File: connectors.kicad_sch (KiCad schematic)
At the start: 23 parts, among them J2 SM08B-SRSS-TB

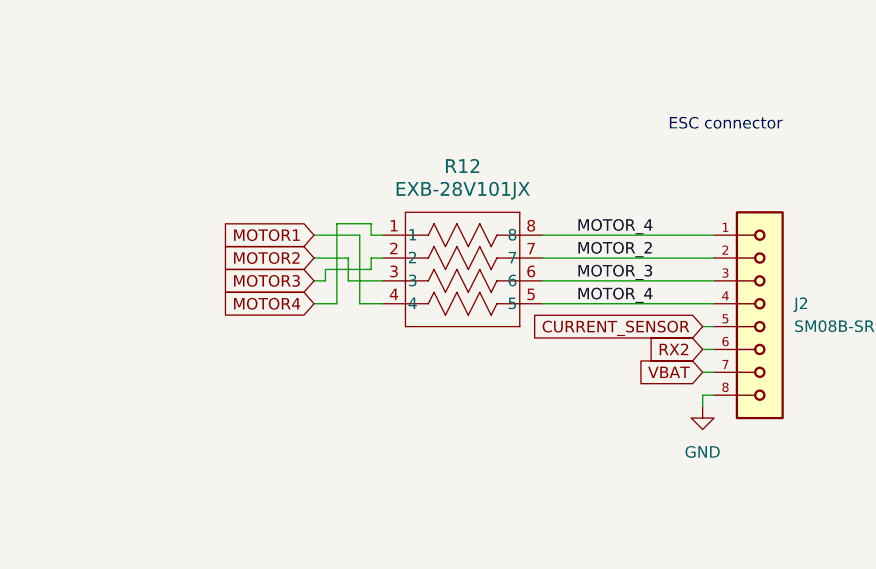
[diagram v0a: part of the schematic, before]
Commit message: routing...
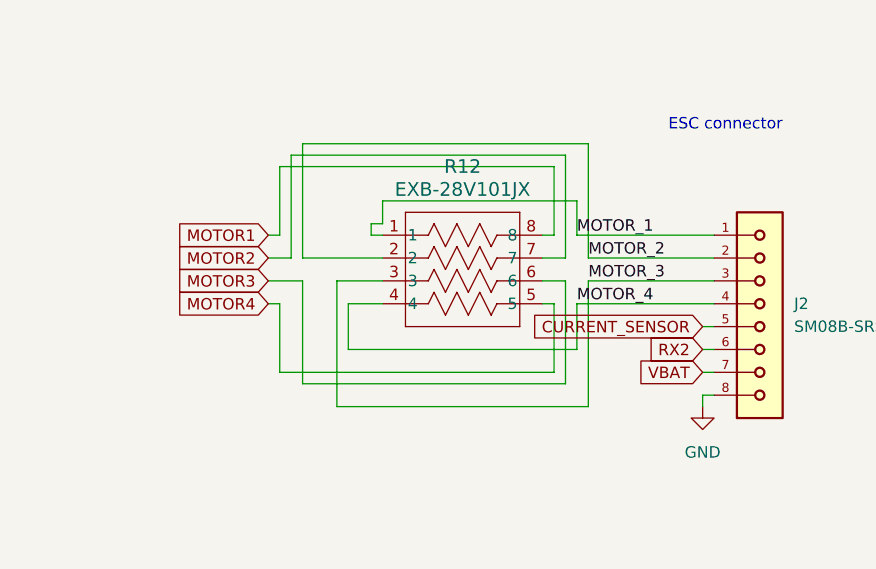
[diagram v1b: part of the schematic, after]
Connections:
- net MOTOR1: now also R12.8; no longer R12.4
- net MOTOR2: now also R12.7; no longer R12.3
- net MOTOR3: now also R12.6; no longer R12.2
- net MOTOR4: now also R12.5; no longer R12.1
- net MOTOR_2: now also R12.2; no longer R12.7
- net MOTOR_3: now also R12.3; no longer R12.6
- net MOTOR_4: now also R12.4; no longer J2.1, R12.5, R12.8
- new net MOTOR_1: J2.1, R12.1

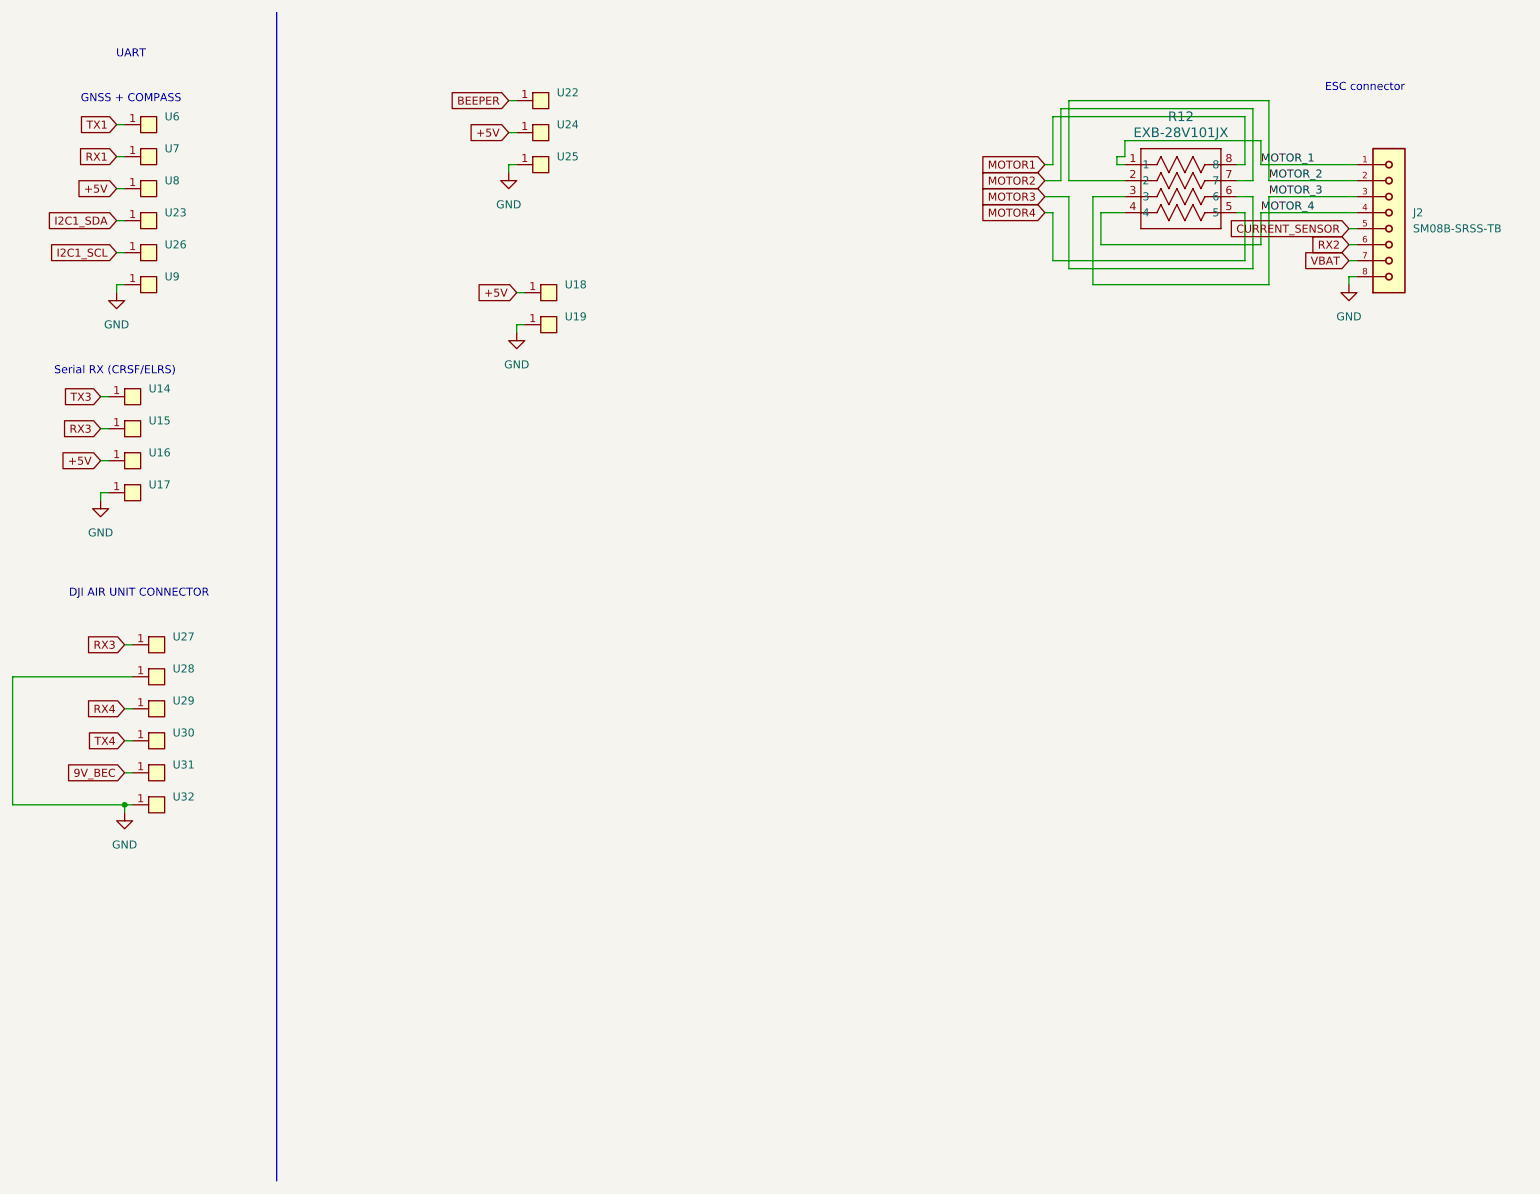
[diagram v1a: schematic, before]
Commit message: routing...
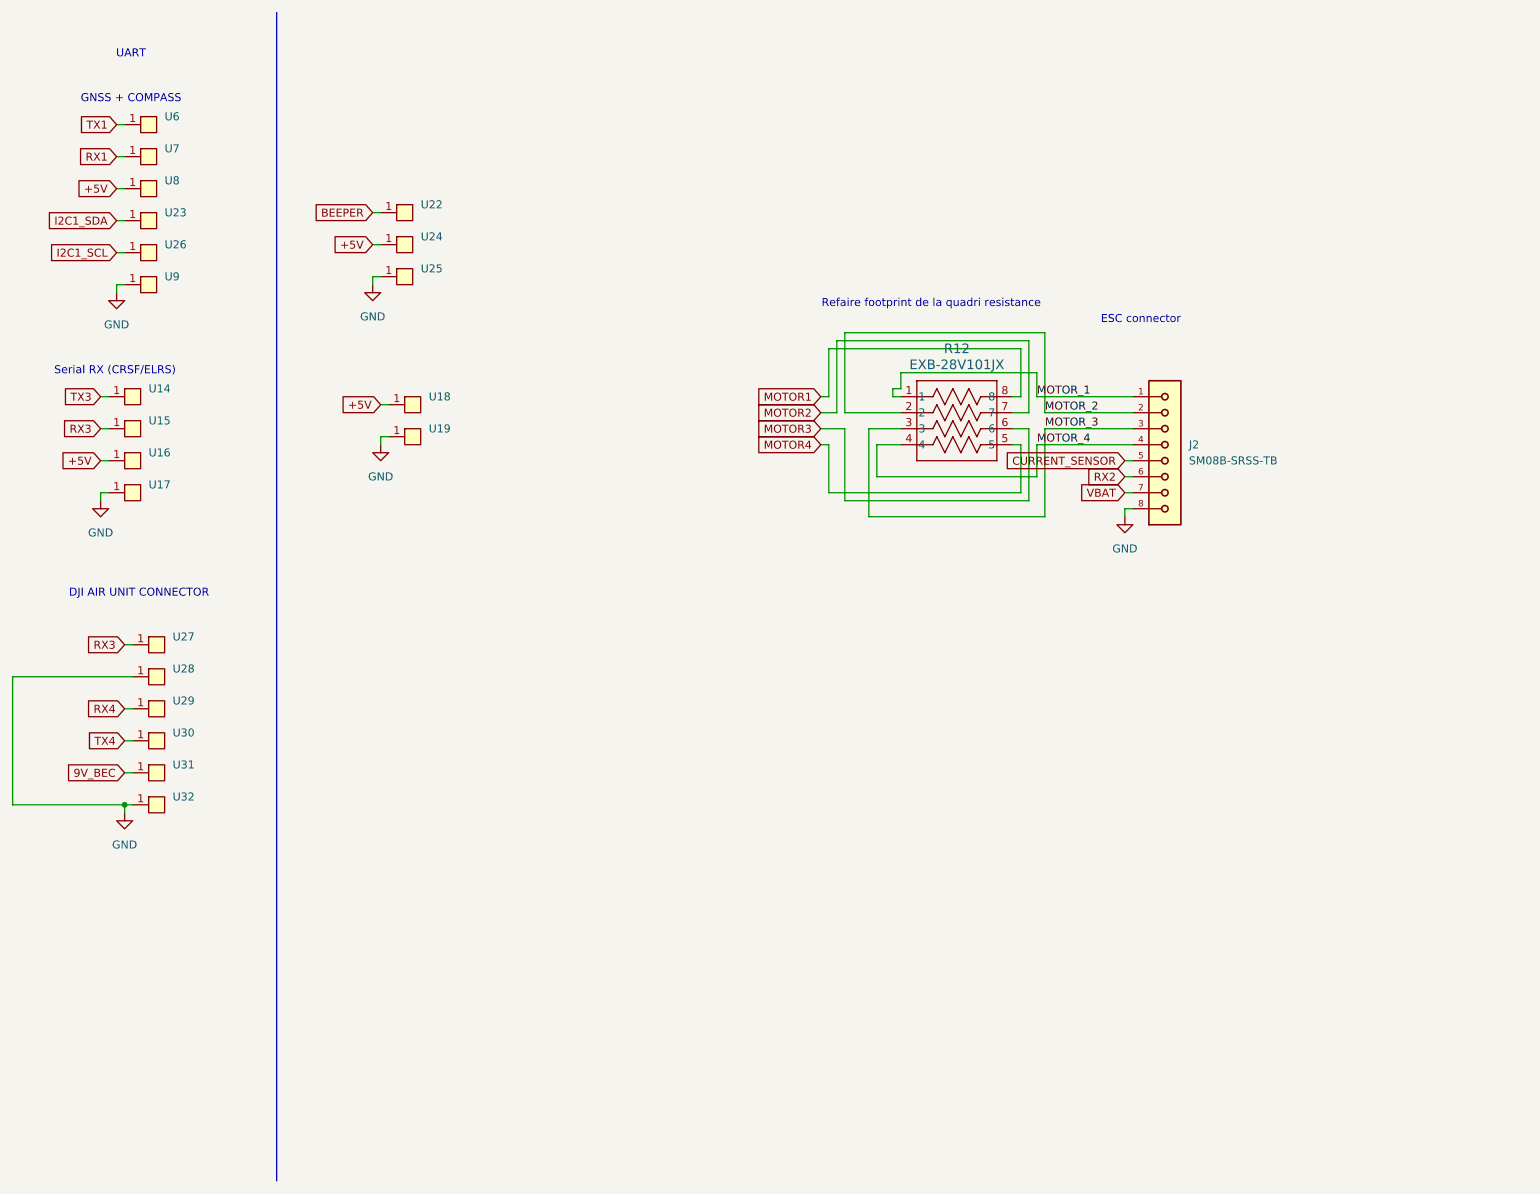
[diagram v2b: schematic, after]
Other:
- note added: "Refaire footprint de la quadri resistance"
- moved on the sheet: J2, R12, U18, U19, U22, U24, U25
